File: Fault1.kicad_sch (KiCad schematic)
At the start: 45 parts

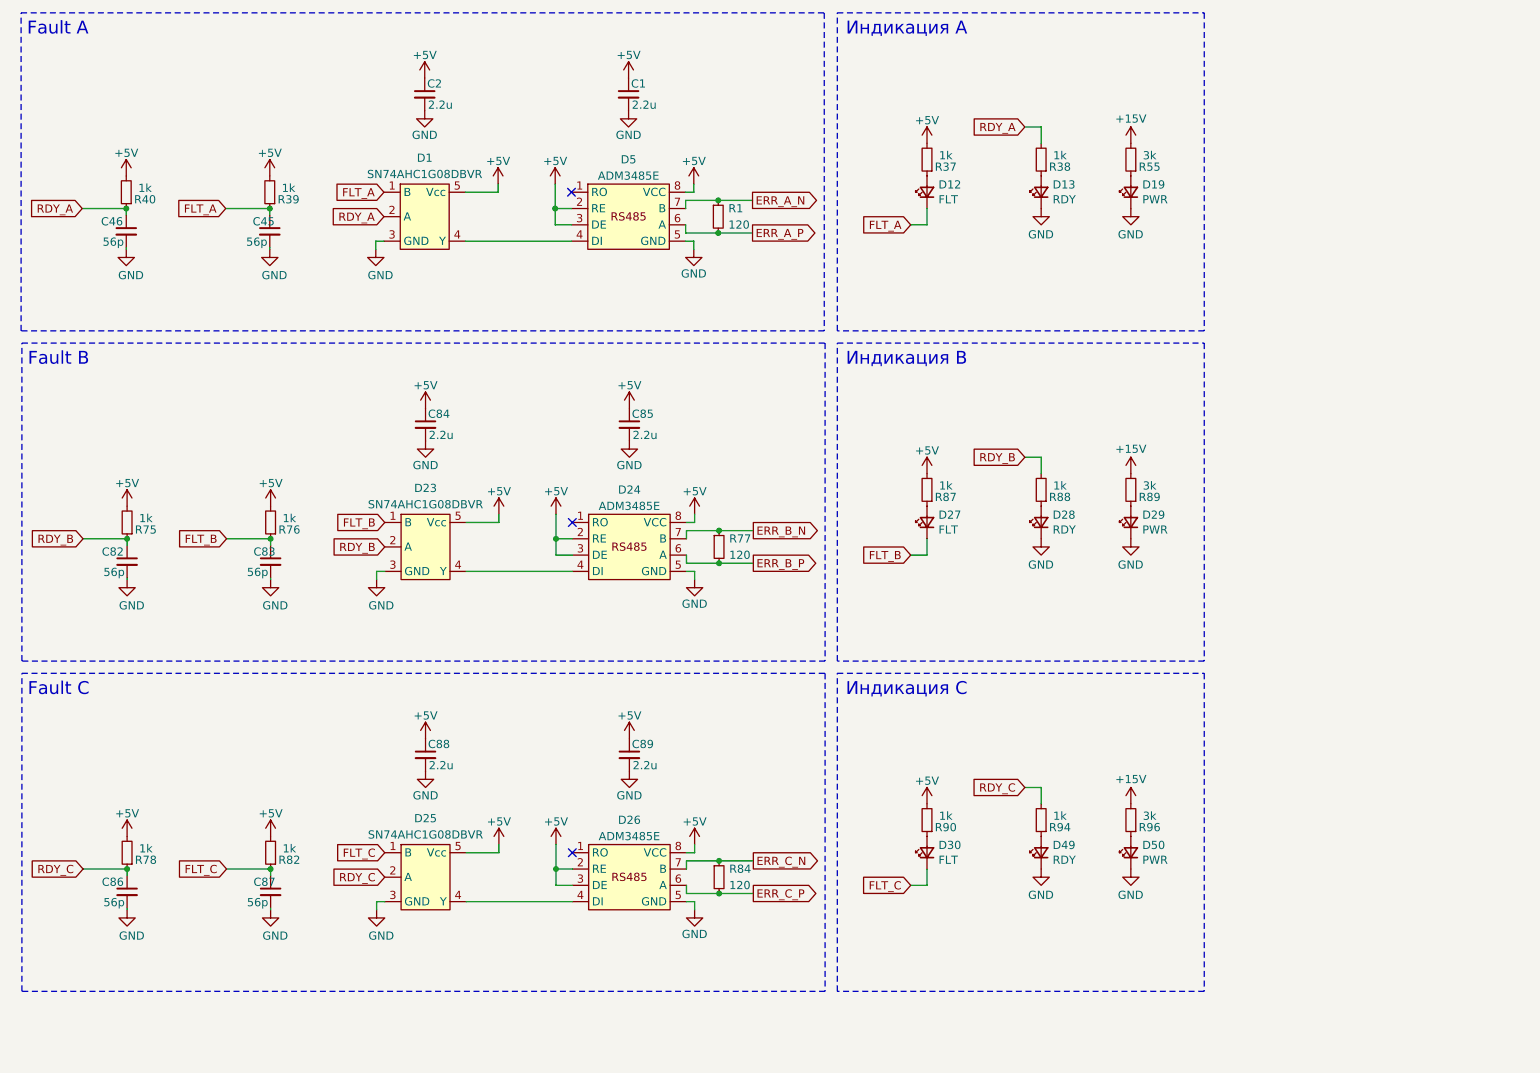
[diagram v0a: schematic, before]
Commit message: VER2.1: добавил СБ и 3D модели в доки
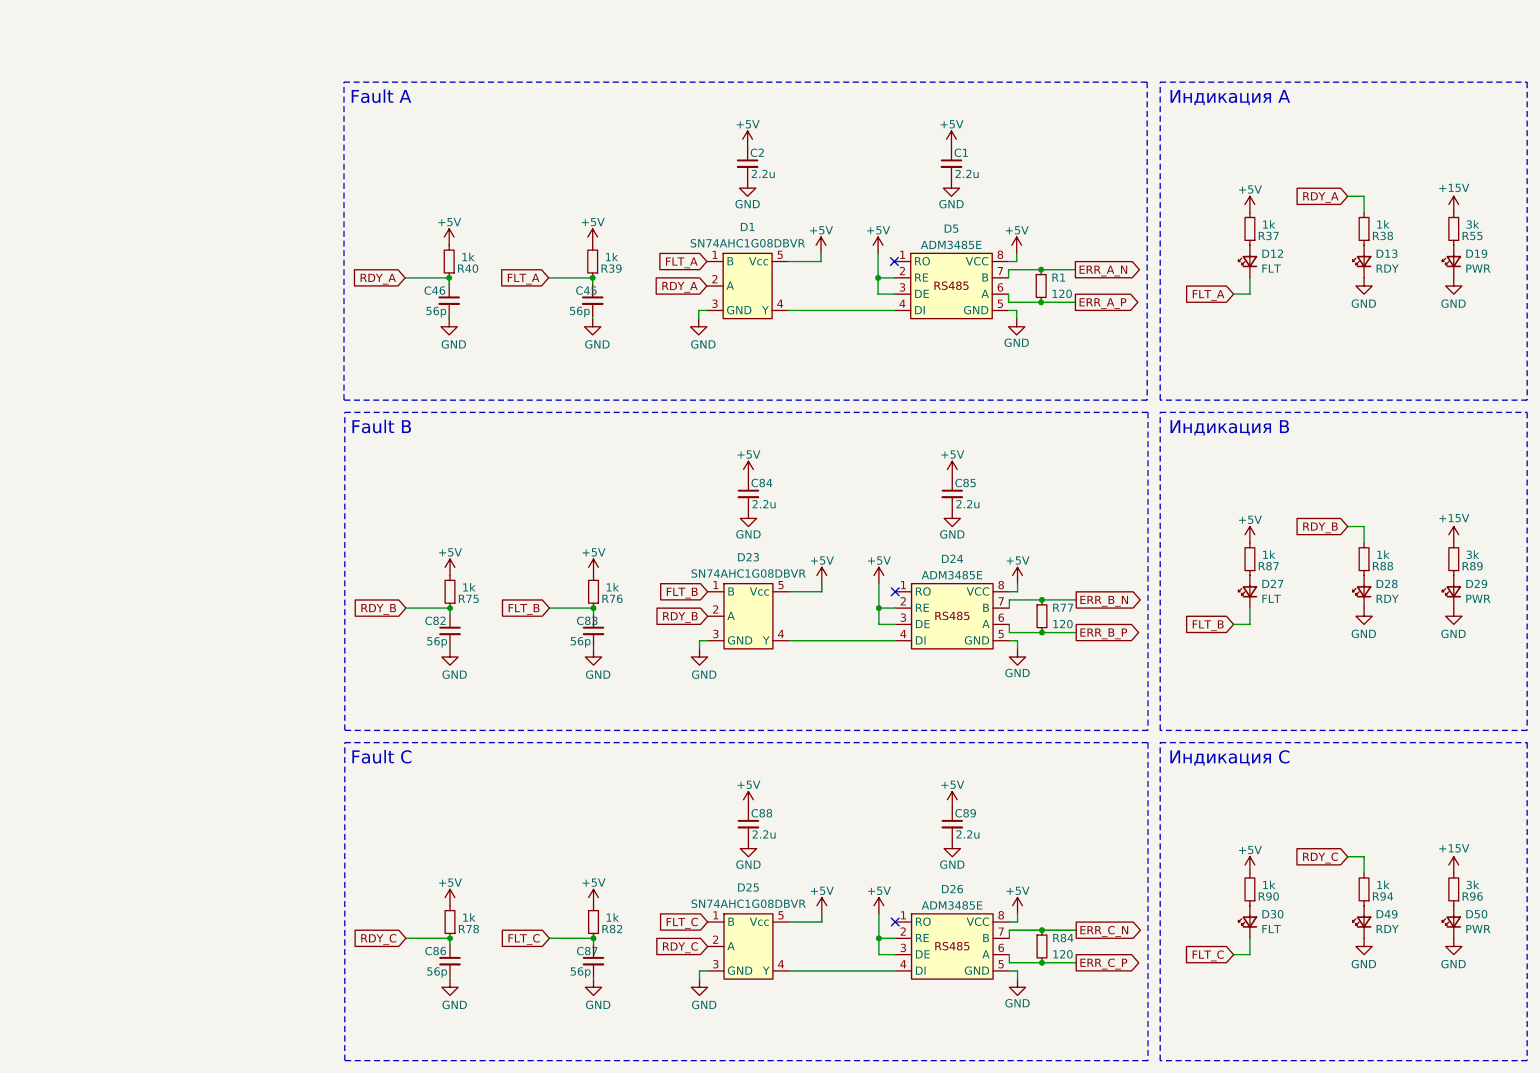
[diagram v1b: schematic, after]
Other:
- moved on the sheet: C1, C2, C45, C46, C82, C83, C84, C85, C86, C87, C88, C89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
